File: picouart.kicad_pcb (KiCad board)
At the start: 2 copper layers, 35 x 17 mm, 20 parts, among them J1 USB, J2 UART, U1 CH340X, U2 AMS1117-3.3, U3 USBLC6-2P6, U4 USBLC6-4SC6

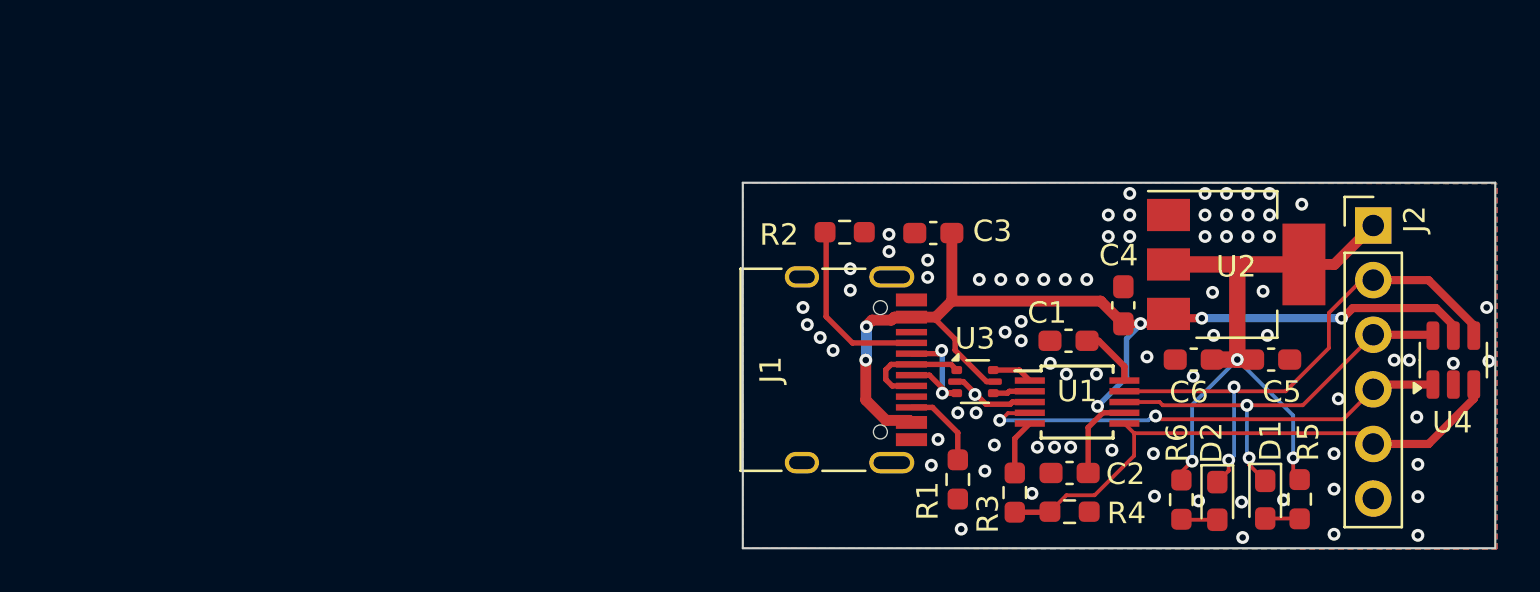
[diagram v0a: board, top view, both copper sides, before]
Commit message: Rev 5
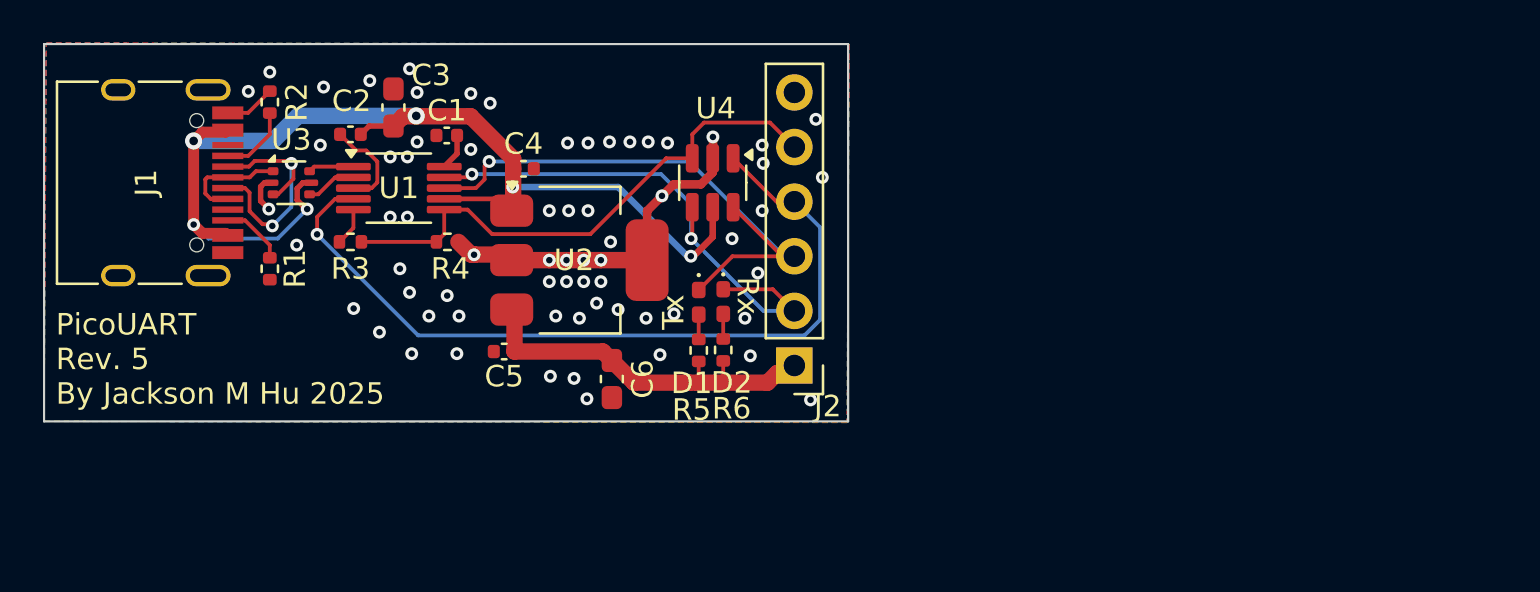
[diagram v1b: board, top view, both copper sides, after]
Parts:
- C1, C2, C4, C5: footprint Capacitor_SMD:C_0603_1608Metric_Pad1.08x0.95mm_HandSolder -> Capacitor_SMD:C_0402_1005Metric
- D1, D2: footprint LED_SMD:LED_0603_1608Metric_Pad1.05x0.95mm_HandSolder -> LED_SMD:LED_0402_1005Metric_Pad0.77x0.64mm_HandSolder
- R1, R2, R3, R4, R5, R6: footprint Resistor_SMD:R_0603_1608Metric_Pad0.98x0.95mm_HandSolder -> Resistor_SMD:R_0402_1005Metric
- U2: value AMS1117-3.3 -> AP7361C-33E
- moved C2 37.0 mm to (104.8, 72.8)
- moved C5 35.7 mm to (111.9, 82.8), turned to 180 degrees
- moved U4 35.4 mm to (121.6, 75.0), turned to -90 degrees
- moved R1 33.5 mm to (101.0, 79.0)
- moved U3 33.1 mm to (102.0, 75.0)
- moved U1 33.1 mm to (107.0, 75.2)
- moved R3 33.0 mm to (104.8, 77.8), turned to 0 degrees
- moved J1 33.0 mm to (95.0, 75.0)
- moved R4 31.5 mm to (109.3, 77.8)
- moved U2 30.6 mm to (115.4, 78.6)
- moved C1 30.5 mm to (109.2, 72.8)
- moved R5 28.8 mm to (121.0, 82.8), turned to 90 degrees
- moved C4 28.6 mm to (112.8, 74.3), turned to 0 degrees
- moved D1 27.9 mm to (121.0, 80.6)
- moved J2 27.7 mm to (125.4, 83.5), turned to 180 degrees
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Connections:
- U2 pad 1: GND -> +5V
- U2 pad 2: +3V3 -> GND
- U2 pad 3: +5V -> +3V3
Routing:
- net GND: track 3.99 -> 25.6 mm, vias 78 -> 67
- net RESET: track 22.6 -> 38.2 mm, vias 2 -> 1
- net +3V3: track 30.2 -> 18.0 mm, vias 3 -> 0
- net TxD: track 19.7 -> 27.9 mm, vias 2 -> 1
- net Net-(J1-CC1): track 8.42 -> 3.36 mm
- net USB_DM_IN: track 6.74 -> 11.7 mm
- net Net-(U1-V3): track 2.88 -> 1.70 mm
- net +5V: track 53.8 -> 52.8 mm
- net Net-(J1-CC2): track 3.90 -> 3.02 mm
- net Net-(U1-CTS): track 2.59 -> 1.77 mm
- net BOOT: track 25.9 -> 25.2 mm
- net USB_DM: track 1.74 -> 2.36 mm
- net RxD: track 25.7 -> 25.1 mm
- net Net-(D2-A): track 1.68 -> 1.17 mm
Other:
- board size 35 x 17 mm -> 37.4 x 17.5 mm
- board text added: "GND BOOT RST TxD RxD +3v3"
- board text added: "PicoUART Rev. 5 By Jackson M Hu 2025"
- board text added: "Rx"
- board text added: "Tx"
- board text removed: "3v3 RxD TxD RST BOOT GND"
- board text removed: "By Jackson M Hu (C) 2024"
- board text removed: "PicoUART Rev 4"
